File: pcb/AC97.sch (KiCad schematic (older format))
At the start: 37 parts, among them J301 JACK_TRRS_6PINS, P301 RCA_2, P302 RCA_2, U301 LM4550, X301 24MHz

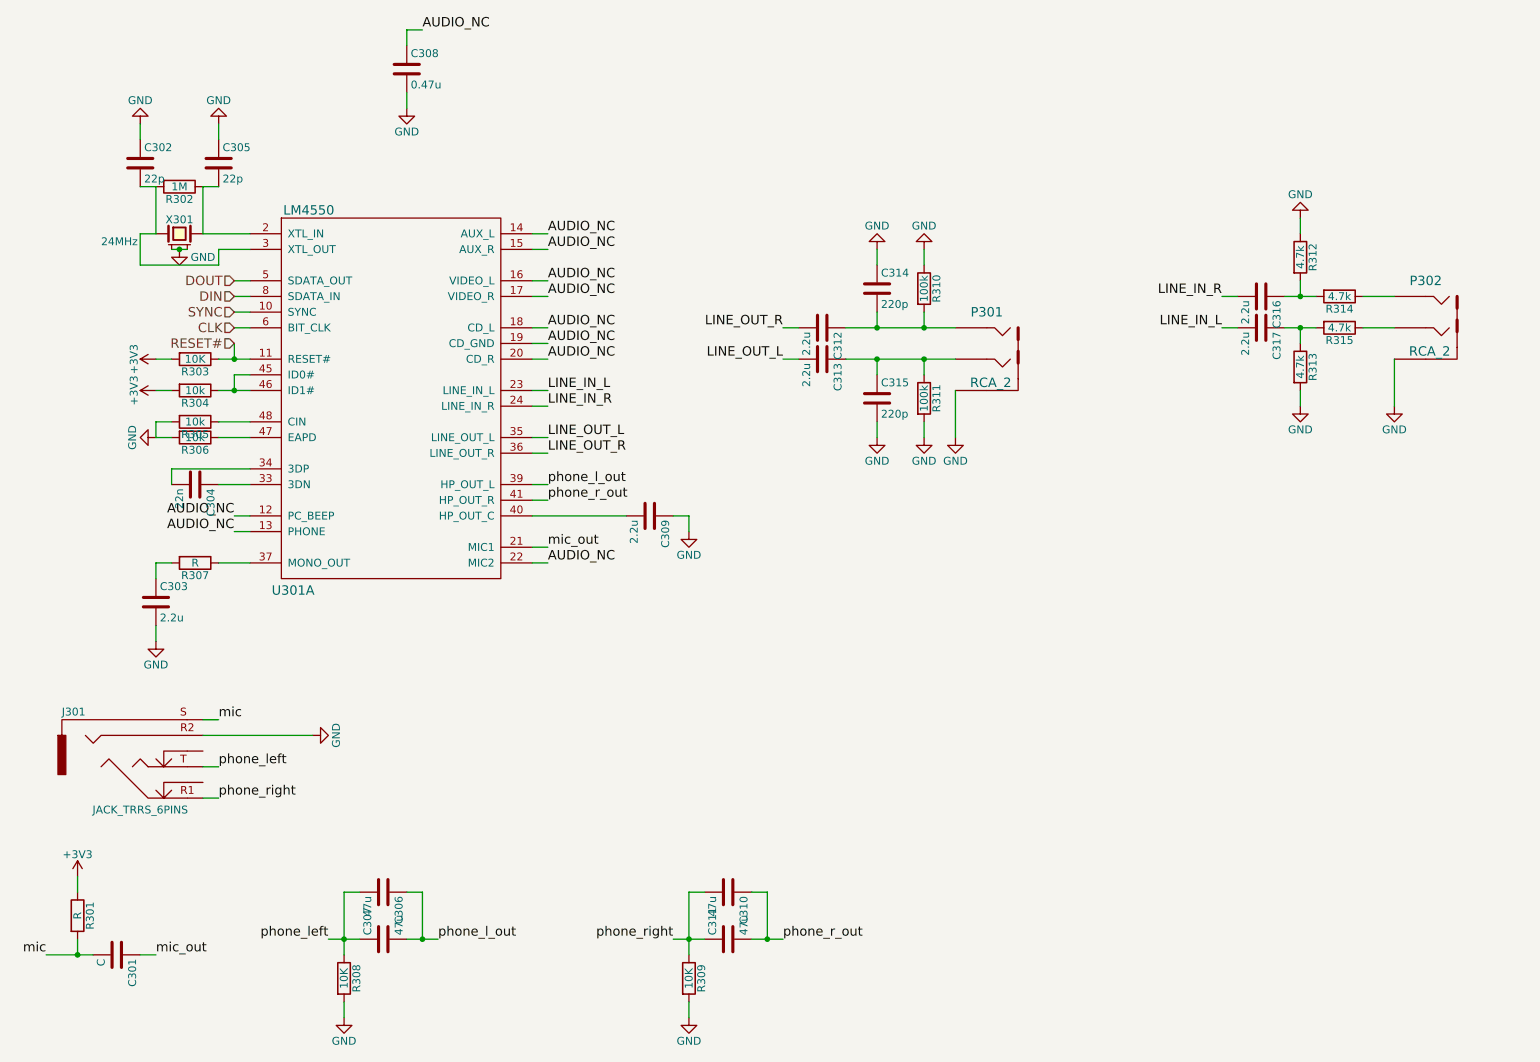
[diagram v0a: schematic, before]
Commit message: added schematic
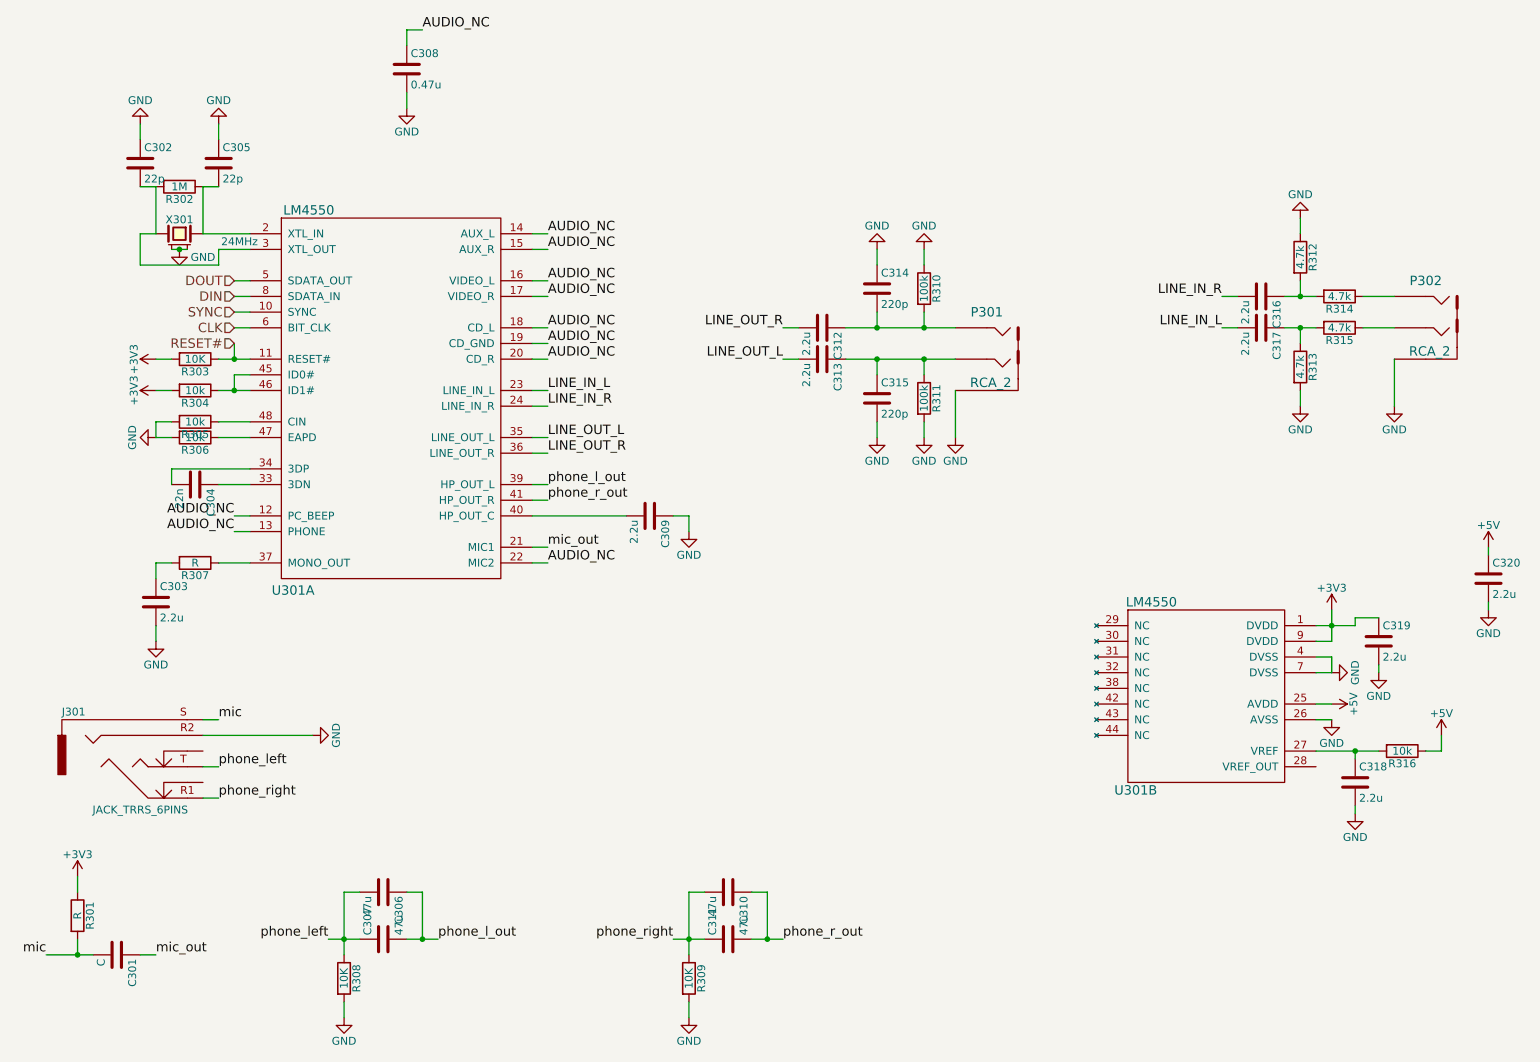
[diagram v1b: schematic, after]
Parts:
- added C318, C319, C320: 2.2u, Capacitors_SMD:C_0805, symbol C
- added R316: 10k, Resistors_SMD:R_0805, symbol R
- added unit 2 of U301
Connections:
- net +3V3: now also C319.1, U301.1 (DVDD), U301.9 (DVDD)
- net GND: now also C318.2, C319.2, C320.2, U301.26 (AVSS), U301.4 (DVSS), U301.7 (DVSS)
- net at C305.2, R302.1, U301.2 (XTL_IN): now also X301.1; no longer X301.3
- net at C302.2, R302.2, U301.3 (XTL_OUT): now also X301.3; no longer X301.1
- new net: C318.1, R316.2, U301.27 (VREF)
- new net +5V: C320.1, R316.1, U301.25 (AVDD)
